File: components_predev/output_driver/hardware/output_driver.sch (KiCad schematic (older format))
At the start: 37 parts

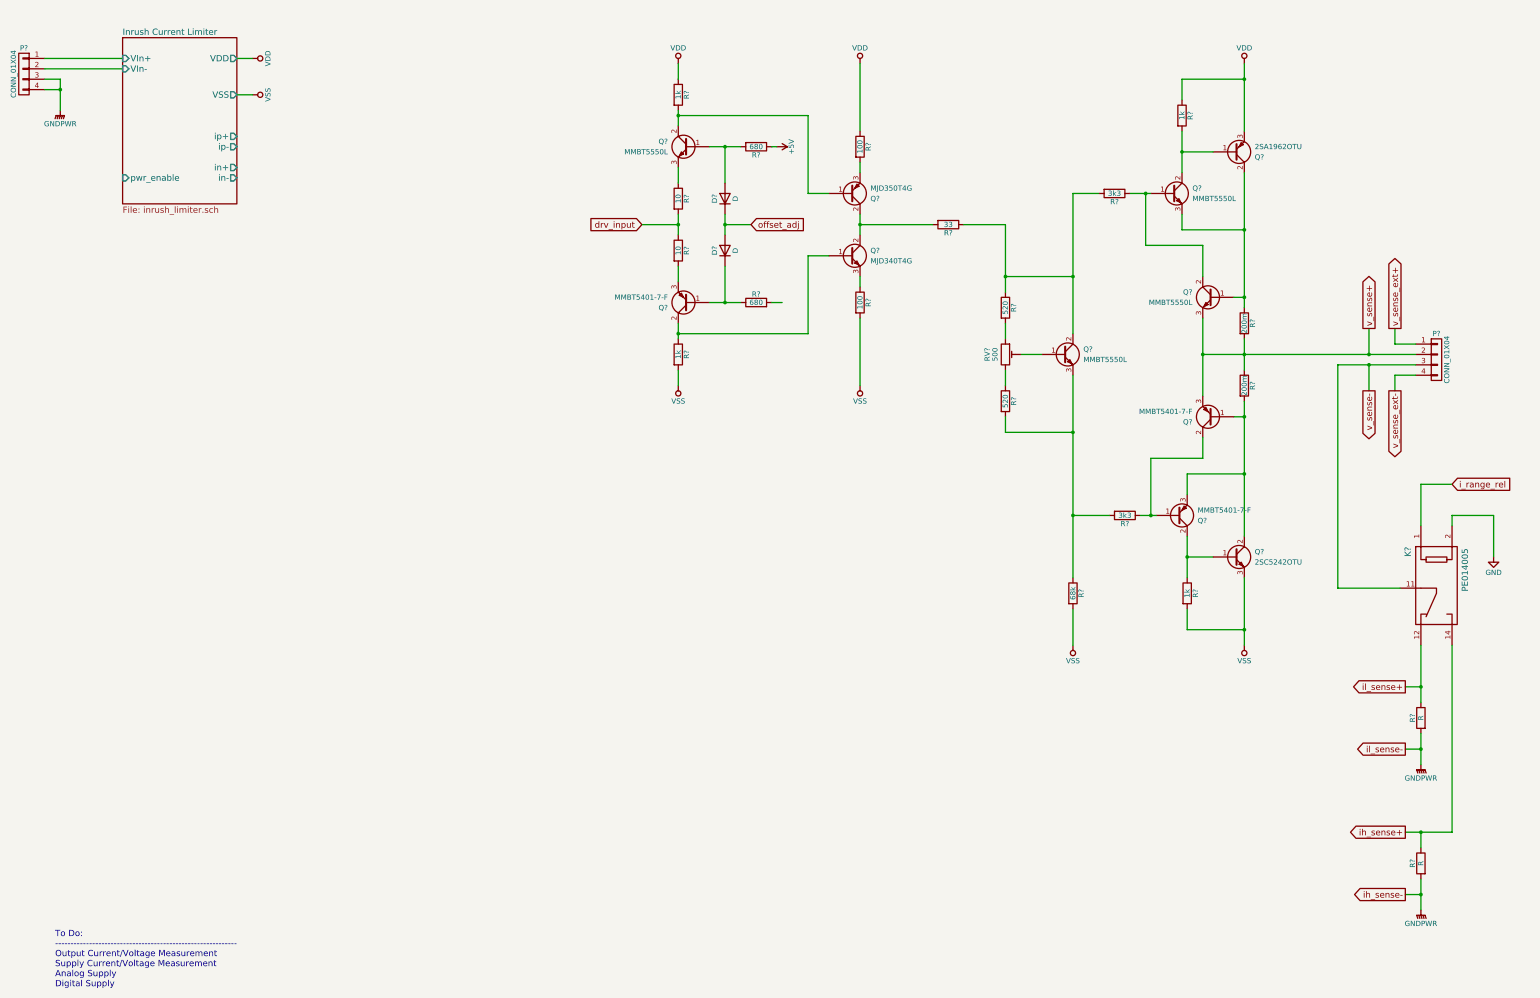
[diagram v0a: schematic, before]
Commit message: Moved output stage to new schematic sheet
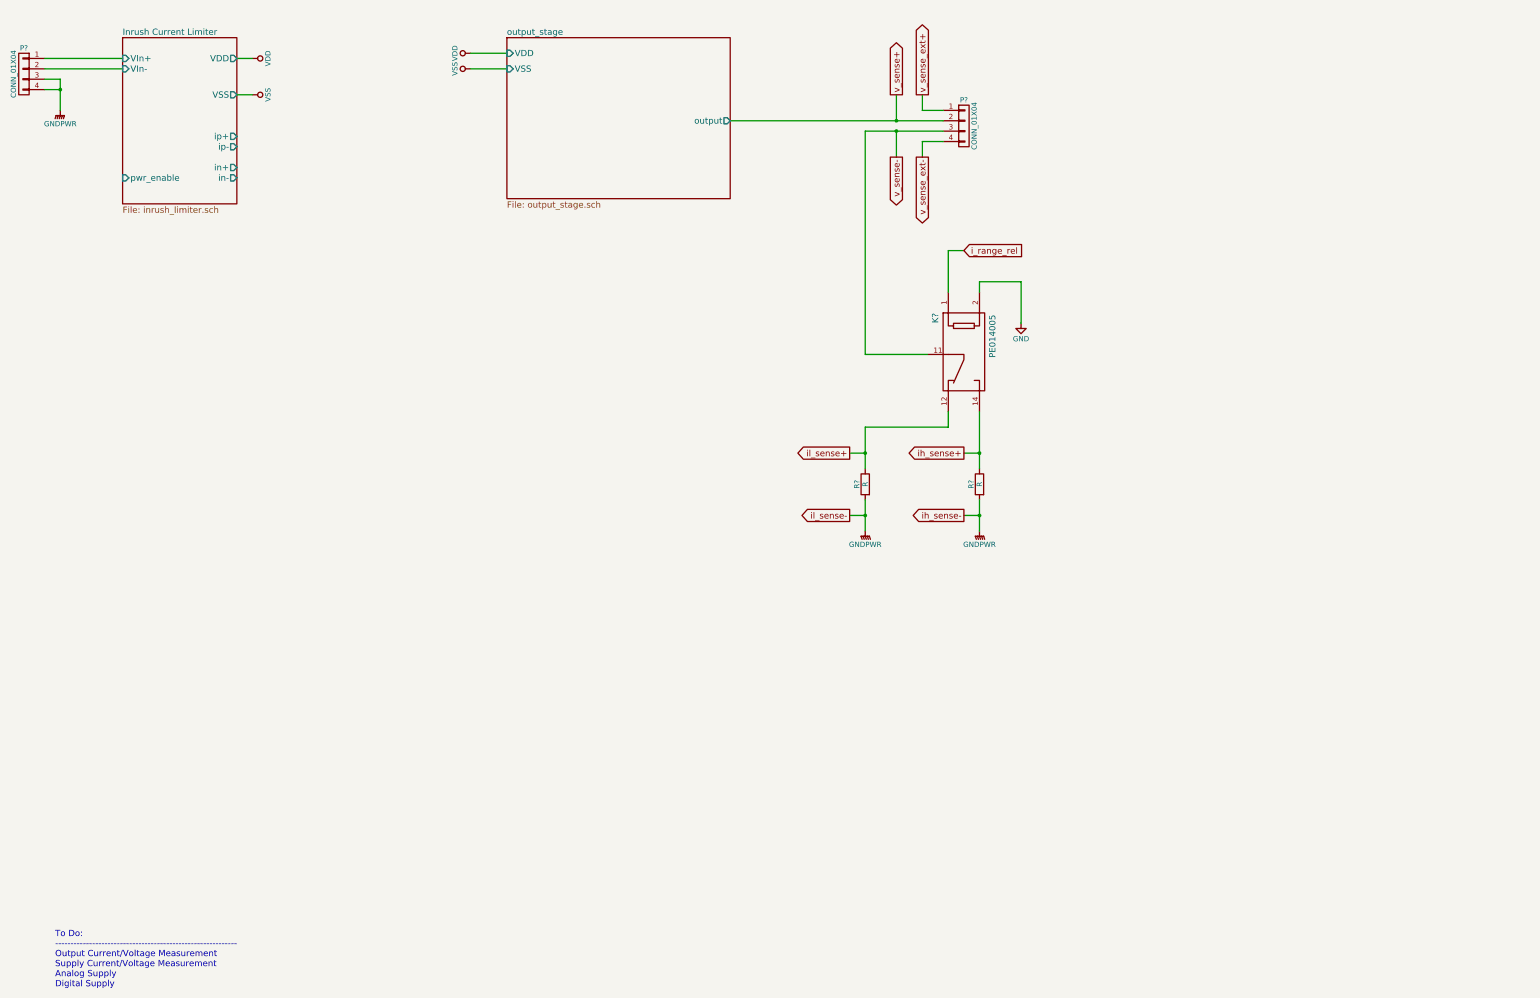
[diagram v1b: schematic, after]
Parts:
- removed D? (x2): D, symbol D
- removed Q?: 2SA1962OTU, symbol Q_PNP_BCE
- removed Q? (x4): MMBT5550L, symbol Q_NPN_BCE
- removed Q? (x3): MMBT5401-7-F, symbol Q_PNP_BCE
- removed Q?: 2SC5242OTU, symbol Q_NPN_BCE
- removed Q?: MJD350T4G, symbol Q_PNP_BCE
- removed Q?: MJD340T4G, symbol Q_NPN_BCE
- removed R? (x4): 1k, symbol R
- removed R? (x2): 200m, symbol R
- removed R? (x2): 3k3, symbol R
- removed R? (x2): 520, symbol R
- removed R?: 68k, symbol R
- removed R?: 33, symbol R
- removed R? (x2): 100, symbol R
- removed R? (x2): 10, symbol R
- removed R? (x2): 680, symbol R
- removed RV?: 500, symbol POT_TRIM
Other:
- moved on the sheet: K?, P?, R?
